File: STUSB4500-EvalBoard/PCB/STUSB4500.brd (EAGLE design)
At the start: 16 x 26 mm, 25 parts

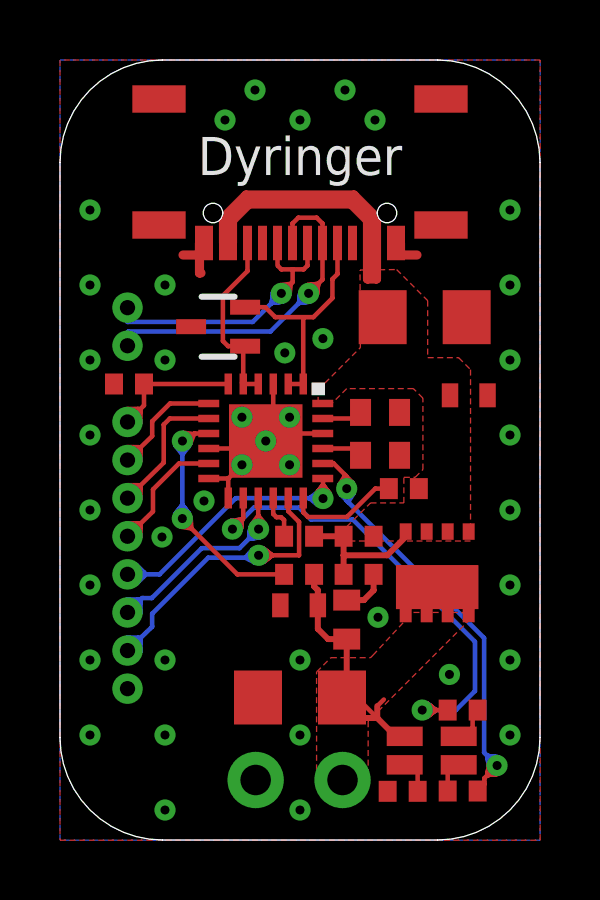
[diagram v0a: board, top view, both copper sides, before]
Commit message: Cleanups in  stusb4500 eval
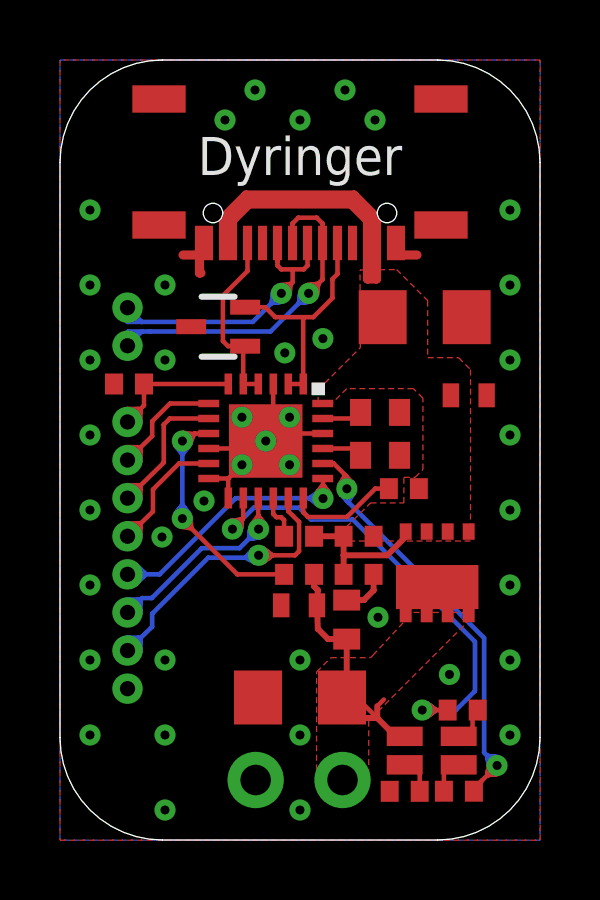
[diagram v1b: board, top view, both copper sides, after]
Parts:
- moved R3 0.13 mm to (13.3, 1.63)
- moved R2 0.07 mm to (11.5, 1.62)
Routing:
- net USB_D+: track 14.3 -> 15.0 mm
- net USB_D-: track 17.6 -> 18.3 mm
